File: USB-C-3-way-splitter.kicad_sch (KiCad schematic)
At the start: 35 parts, among them J1 USB_C_Receptacle_USB2.0, J2 Conn_01x04, J3 Conn_01x04, J4 Conn_01x04, U1 LM393, U2 SiP32509

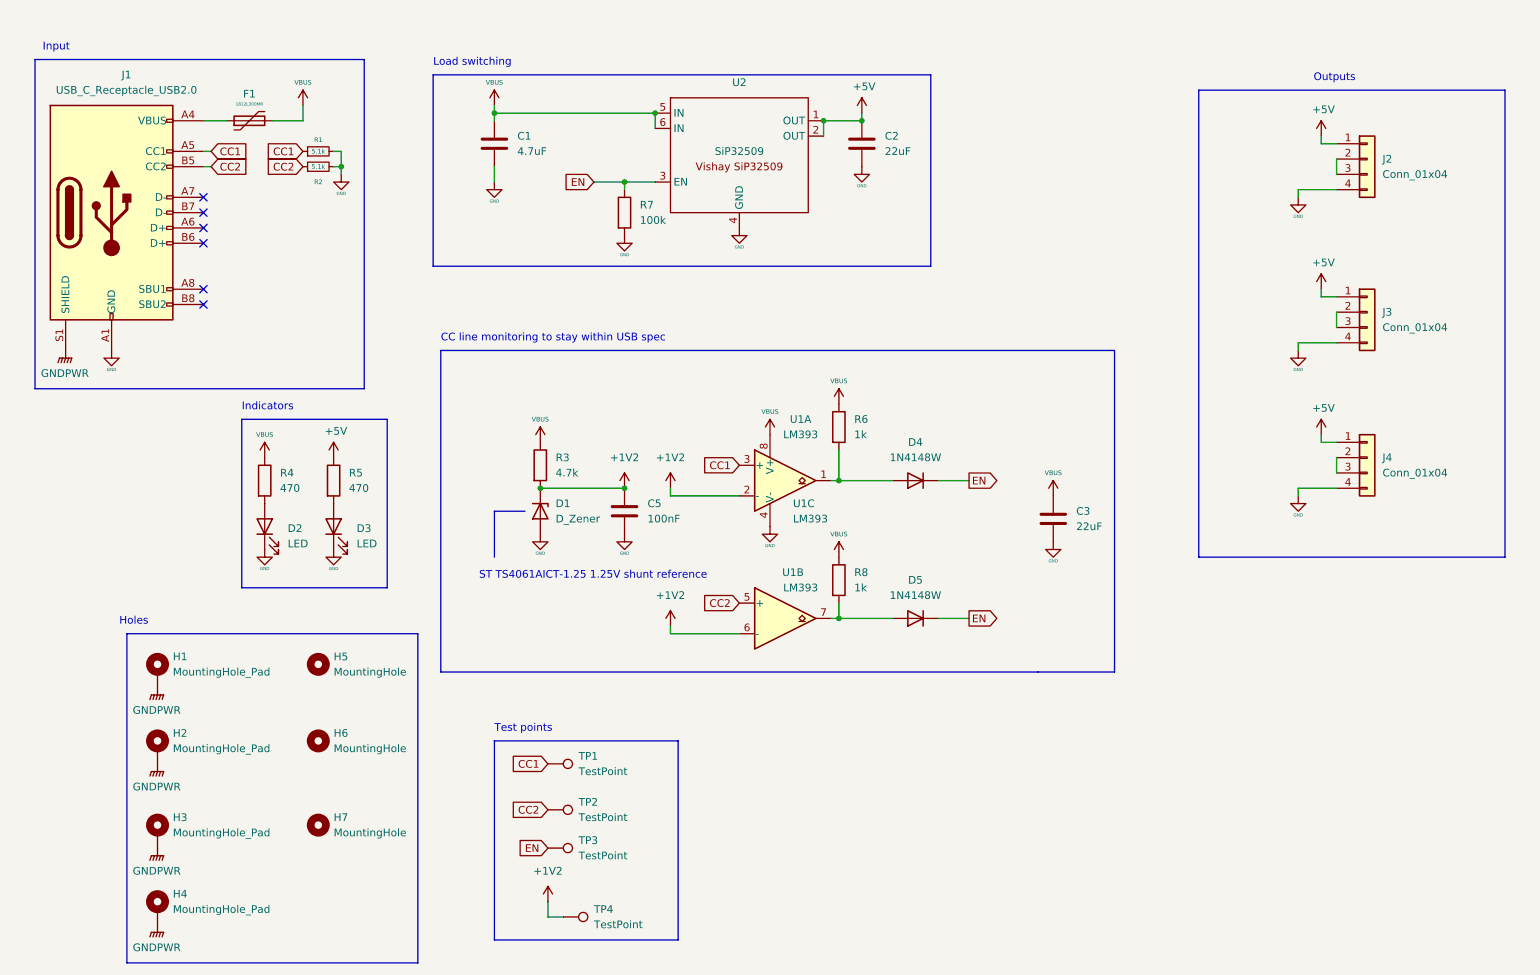
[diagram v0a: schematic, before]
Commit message: Some organization and updates
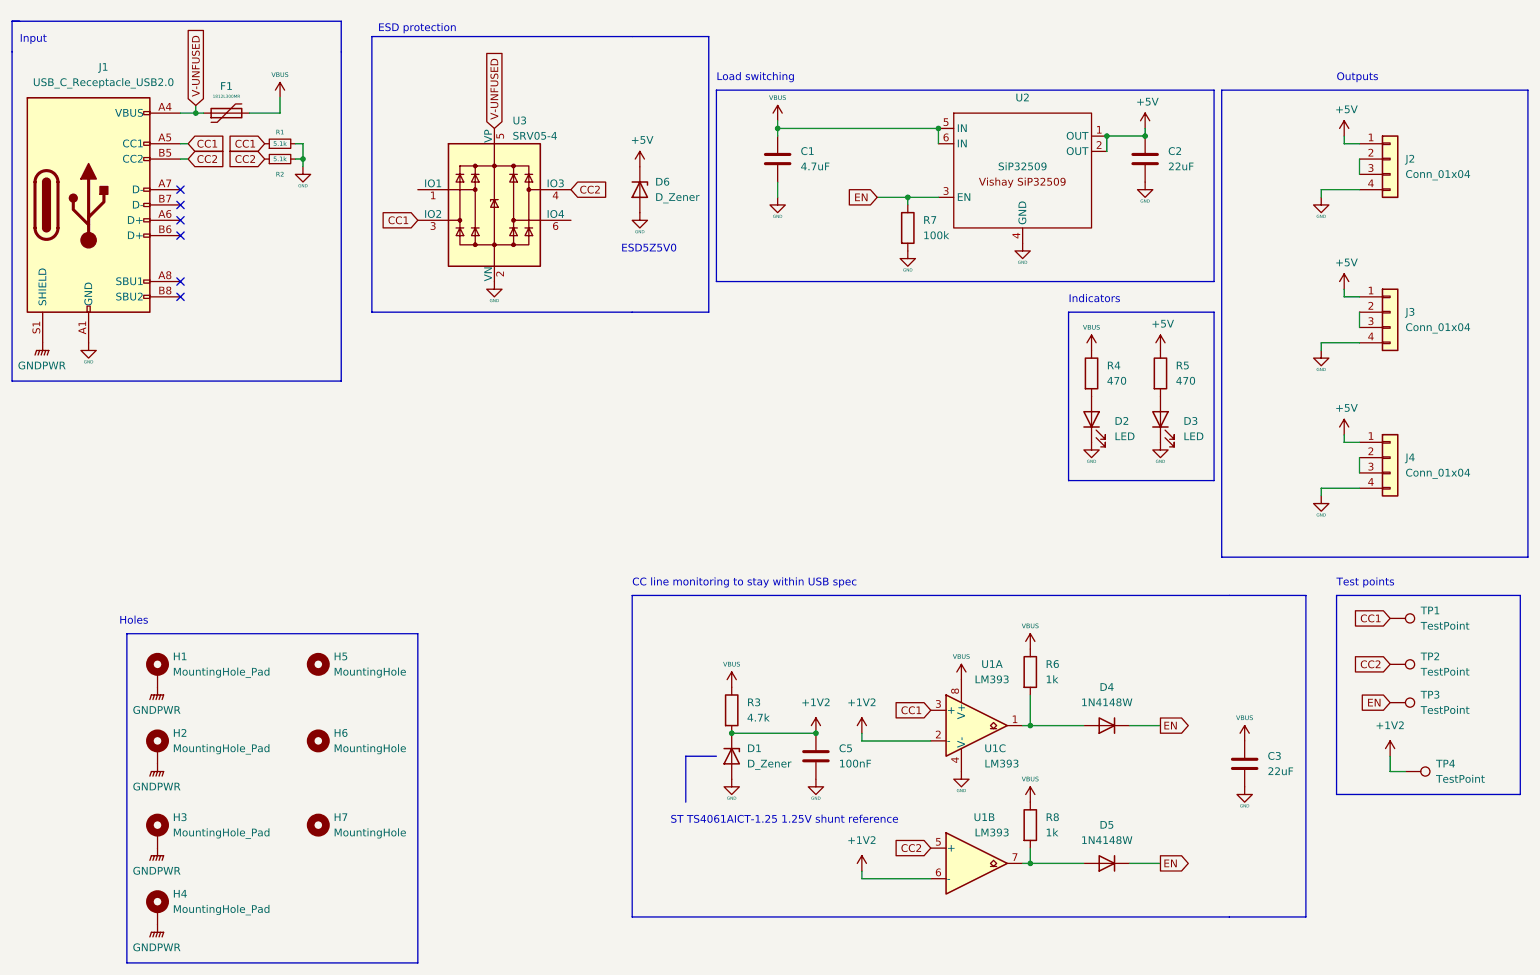
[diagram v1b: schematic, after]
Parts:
- added D6: D_Zener, Diode_SMD:D_SOD-523, symbol Device:D_Zener
- added U3: SRV05-4, Package_TO_SOT_SMD:SOT-23-6, symbol Power_Protection:SRV05-4
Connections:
- net +5V: now also D6.1 (K)
- net CC1: now also U3.3 (IO2)
- net CC2: now also U3.4 (IO3)
- net GND: now also D6.2 (A), U3.2 (VN)
- net V-UNFUSED: now reaches F1.1, J1.A4 (VBUS), J1.A9 (VBUS), J1.B4 (VBUS), J1.B9 (VBUS)
- net V-UNFUSED: now also U3.5 (VP)
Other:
- note added: "ESD protection"
- note added: "ESD5Z5V0"
- moved on the sheet: C1, C2, C3, C5, D1, D2, D3, D4, D5, F1, J1, J2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
